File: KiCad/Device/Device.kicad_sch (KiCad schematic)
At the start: 4 parts, among them IC1 ATTINY167-XUR, J1 Conn_02x04_Odd_Even

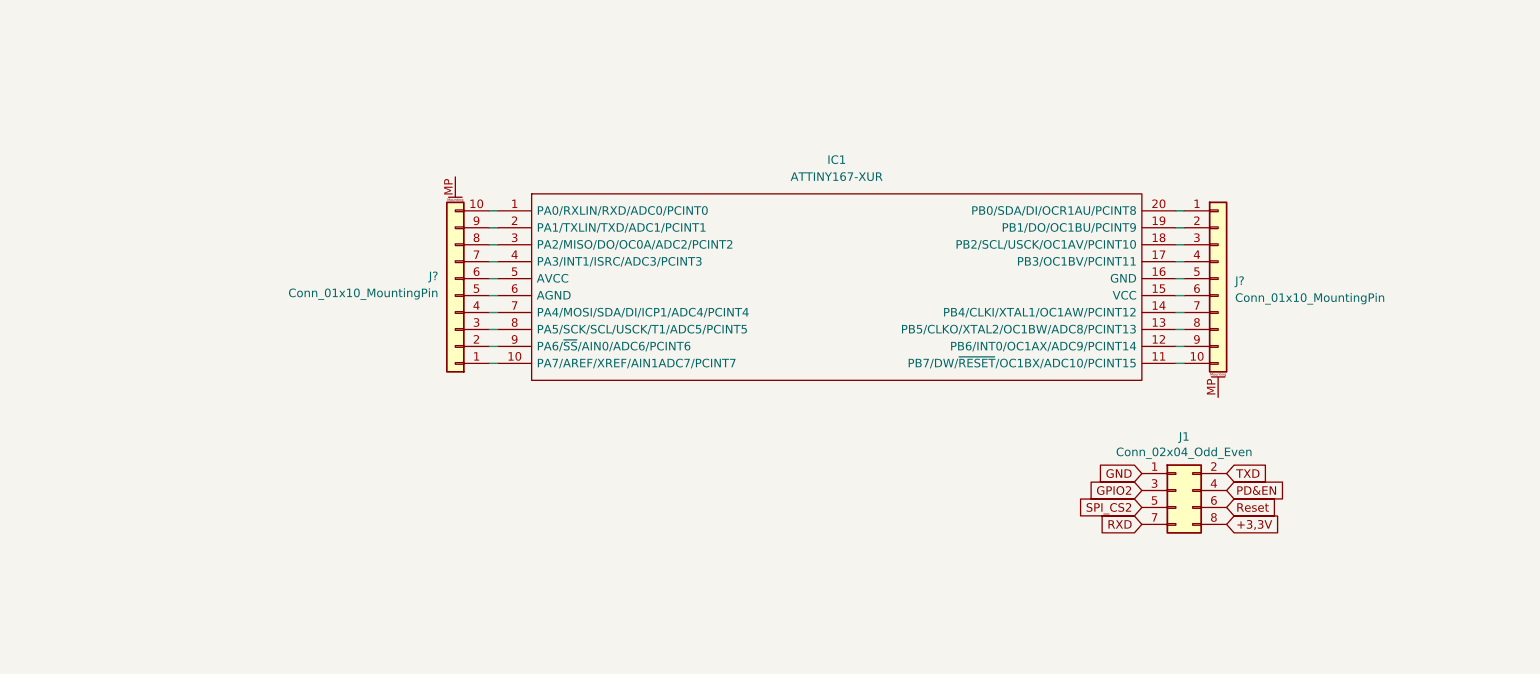
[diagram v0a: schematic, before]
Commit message: device tilføjelse
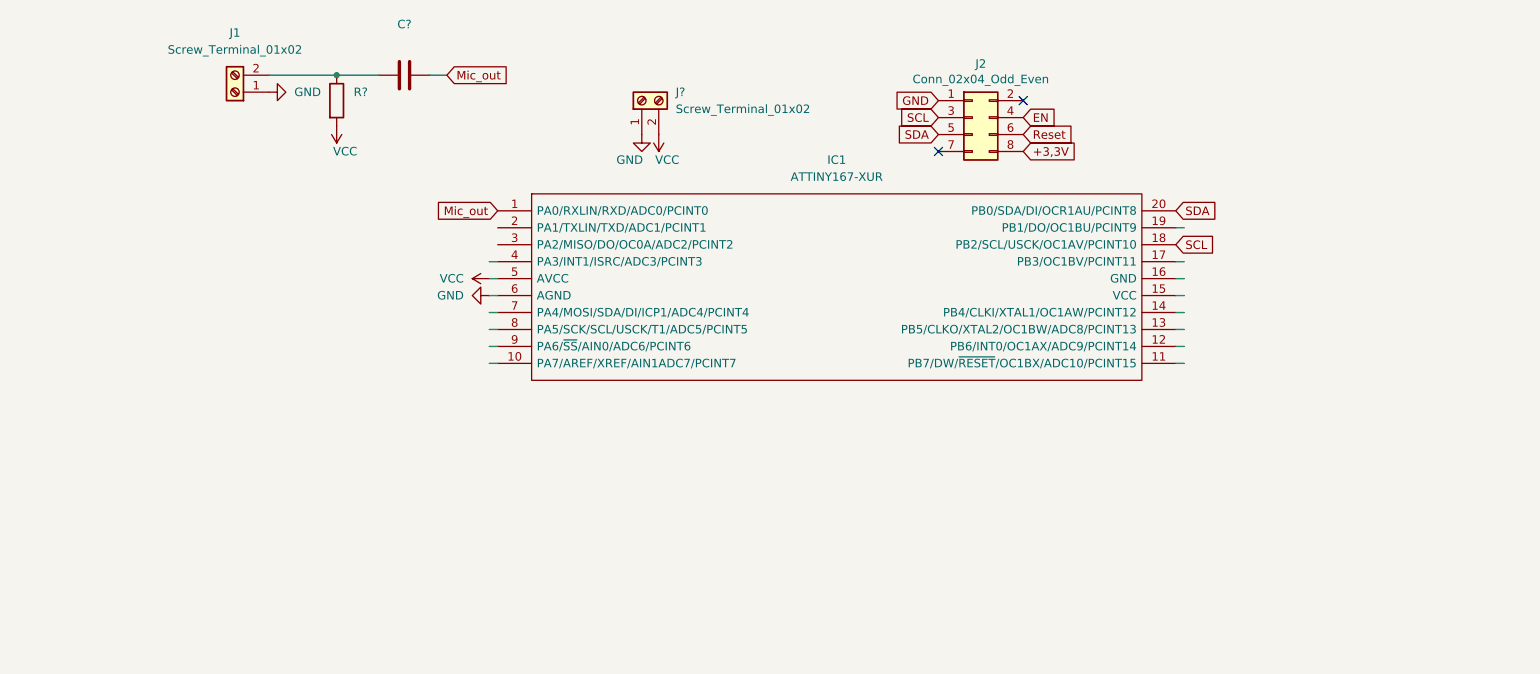
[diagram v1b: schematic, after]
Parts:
- removed J? (x2): Conn_01x10_MountingPin, Connector_PinHeader_2.54mm:PinHeader_1x10_P2.54mm_Vertical, symbol Connector_Generic_MountingPin:Conn_01x10_MountingPin
- added C?: (no value), symbol Device:C
- added J1, J?: Screw_Terminal_01x02, symbol Connector:Screw_Terminal_01x02
- added R?: (no value), symbol Device:R
- renumbered J1 to J2
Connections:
- net GPIO2 is gone; now on net SCL: J2.3 (Pin_3)
- net SPI_CS2 is gone; now on net SDA: J2.5 (Pin_5)
- net GND: now also IC1.6 (AGND), J1.1 (Pin_1), J?.1 (Pin_1)
- net Mic_out: now reaches IC1.1 (PA0/RXLIN/RXD/ADC0/PCINT0)
- net Mic_out: now also C?.2
- net VCC: now reaches IC1.5 (AVCC)
- net VCC: now also J?.2 (Pin_2), R?.2
- net SDA: now reaches IC1.20 (PB0/SDA/DI/OCR1AU/PCINT8)
- net SCL: now reaches IC1.18 (PB2/SCL/USCK/OC1AV/PCINT10)
- net PD&EN renamed EN
- net RXD: no longer names the net of J2.7 (Pin_7)
- net TXD: no longer names the net of J2.2 (Pin_2)
- new net: C?.1, J1.2 (Pin_2), R?.1
- no-connect marks 0 -> 2
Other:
- moved on the sheet: J2

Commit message: Device tilføjelser
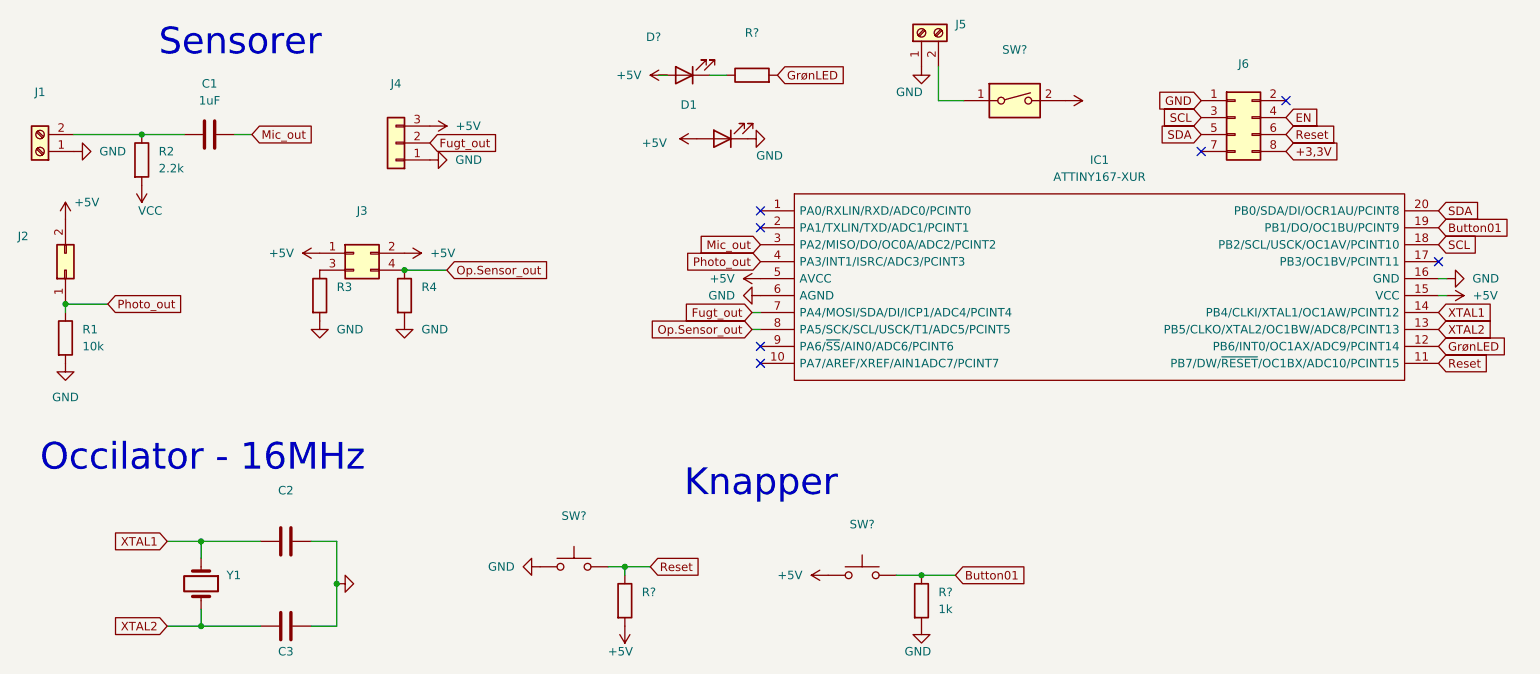
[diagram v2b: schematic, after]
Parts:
- added C2, C3: (no value), symbol Device:C
- added D1, D?: (no value), symbol Device:LED
- added J2: (no value), symbol Connector_Generic:Conn_02x01
- added J3: (no value), symbol Connector_Generic:Conn_02x02_Odd_Even
- added J4: (no value), symbol Connector_Generic:Conn_01x03
- added R1: 10k, symbol Device:R
- added R3, R4, R? (x2): (no value), symbol Device:R
- added R?: 1k, symbol Device:R
- added SW?: (no value), symbol Switch:SW_DIP_x01
- added SW?: (no value), Button_Switch_SMD:SW_MEC_5GSH9, symbol Switch:SW_MEC_5G
- added SW?: (no value), symbol Switch:SW_MEC_5G
- added Y1: (no value), symbol Device:Crystal
- C1: renamed from C?; value (none) -> 1uF
- J1: value Screw_Terminal_01x02 -> (none)
- J5: renamed from J?; value Screw_Terminal_01x02 -> (none)
- J6: renamed from J2; value Conn_02x04_Odd_Even -> (none)
- R2: renamed from R?; value (none) -> 2.2k
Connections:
- net GND: now also IC1.16 (GND), C2.2, C3.2, D1.1 (K), J4.1 (Pin_1), R1.2, R3.2, R4.2, R?.2, SW?.1 (A), SW?.2 (A)
- net Mic_out: now also IC1.3 (PA2/MISO/DO/OC0A/ADC2/PCINT2); no longer IC1.1 (PA0/RXLIN/RXD/ADC0/PCINT0)
- net Reset: now also IC1.11 (PB7/DW/~{RESET}/OC1BX/ADC10/PCINT15), R?.1, SW?.3 (B), SW?.4 (B)
- net VCC: no longer IC1.5 (AVCC), J5.2 (Pin_2)
- net GrønLED: now reaches IC1.12 (PB6/INT0/OC1AX/ADC9/PCINT14)
- net GrønLED: now also R?.2
- net XTAL2: now reaches IC1.13 (PB5/CLKO/XTAL2/OC1BW/ADC8/PCINT13)
- net XTAL2: now also C3.1, Y1.2
- net XTAL1: now reaches IC1.14 (PB4/CLKI/XTAL1/OC1AW/PCINT12)
- net XTAL1: now also C2.1, Y1.1
- net +5V: now reaches IC1.15 (VCC)
- net +5V: now also IC1.5 (AVCC), D1.2 (A), D?.2 (A), J2.2 (Pin_2), J3.1 (Pin_1), J3.2 (Pin_2), J4.3 (Pin_3), R?.2, SW?.1 (A), SW?.2, SW?.2 (A)
- net Button01: now reaches IC1.19 (PB1/DO/OC1BU/PCINT9)
- net Button01: now also R?.1, SW?.3 (B), SW?.4 (B)
- net Photo_out: now reaches IC1.4 (PA3/INT1/ISRC/ADC3/PCINT3)
- net Photo_out: now also J2.1 (Pin_1), R1.1
- net Fugt_out: now reaches IC1.7 (PA4/MOSI/SDA/DI/ICP1/ADC4/PCINT4)
- net Fugt_out: now also J4.2 (Pin_2)
- net Op.Sensor_out: now reaches IC1.8 (PA5/SCK/SCL/USCK/T1/ADC5/PCINT5)
- net Op.Sensor_out: now also J3.4 (Pin_4), R4.1
- new net: J5.2 (Pin_2), SW?.1
- new net: D?.1 (K), R?.1
- new net: J3.3 (Pin_3), R3.1
- no-connect marks 2 -> 7
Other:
- note added: "Knapper"
- note added: "Occilator - 16MHz"
- note added: "Sensorer"
- moved on the sheet: C1, IC1, J1, J5, J6, R2
